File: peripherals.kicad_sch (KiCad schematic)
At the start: 67 parts, among them J402 Amph 10118193-0001LF, J403 Conn_02x20, J404 Molex 1040310811, J405 Amph 10118193-0001LF, U1 TPD2EUSB30, U401 FT230XQ, U402 TLV62569DRL, U403 MX25L1606, U404 TLV62569DRL, U405 TLV62569DRL, U406 TLV75801PDRV, X401 XO32

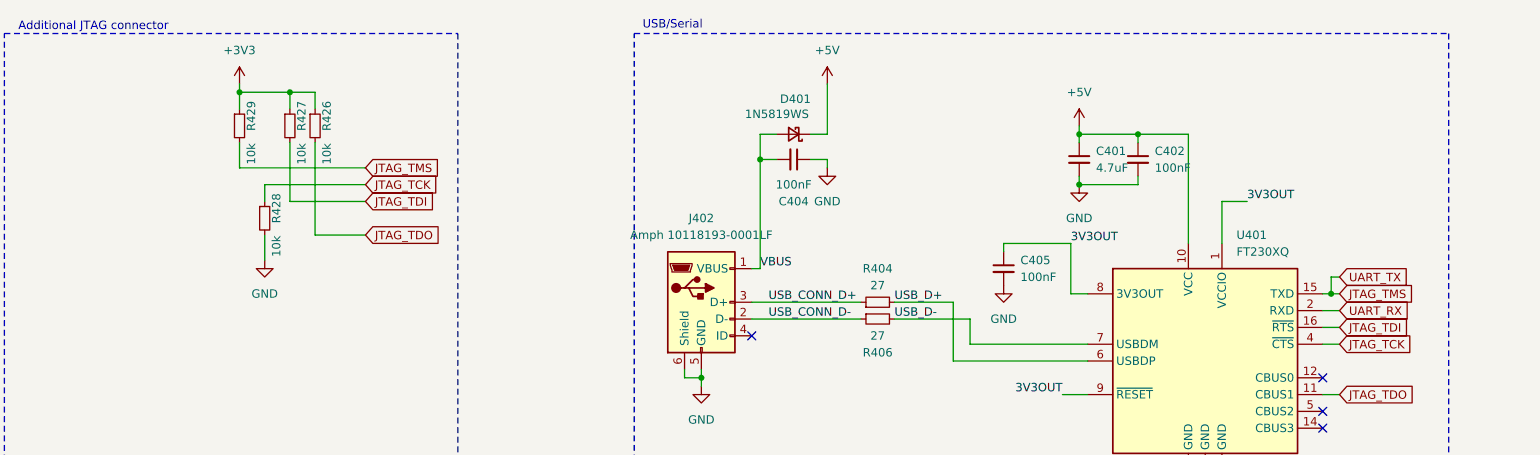
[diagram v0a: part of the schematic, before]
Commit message: Minor fixes
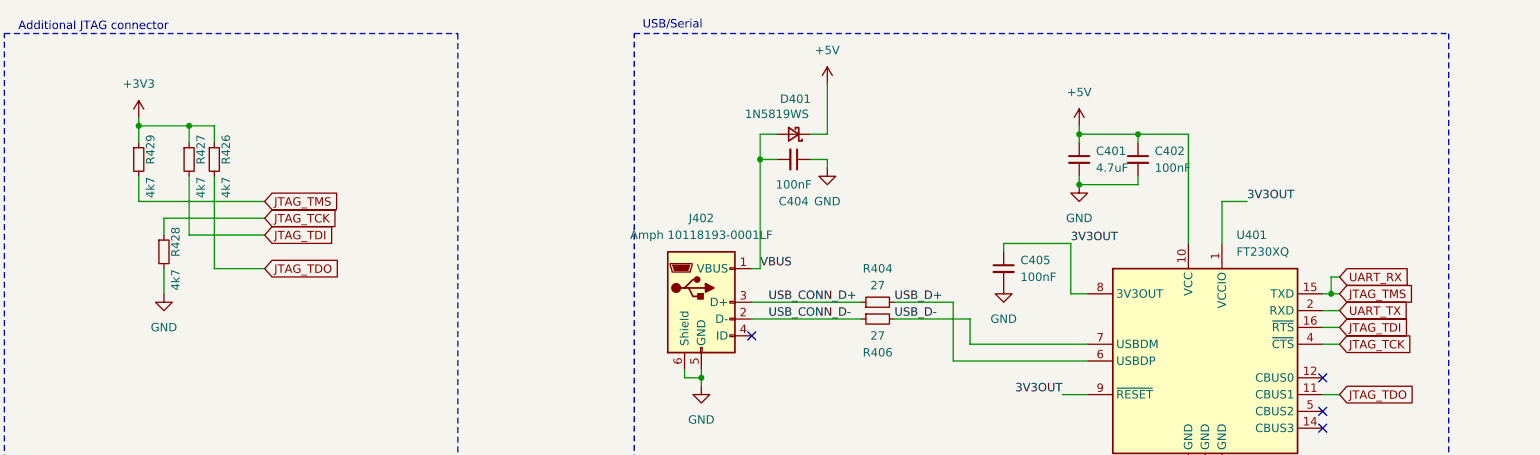
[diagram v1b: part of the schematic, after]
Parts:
- R426, R427, R428, R429: value 10k -> 4k7; MPN C25744 -> (none)
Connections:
- net UART_RX renamed UART_TX
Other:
- moved on the sheet: R426, R427, R428, R429
